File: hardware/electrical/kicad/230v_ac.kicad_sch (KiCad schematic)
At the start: 0 parts

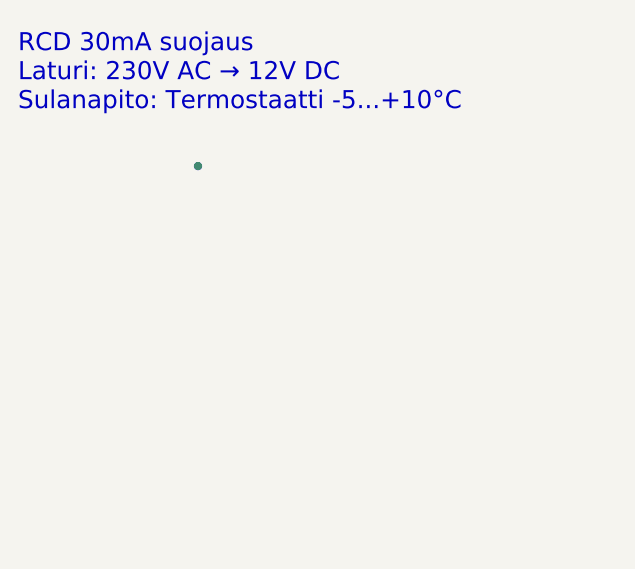
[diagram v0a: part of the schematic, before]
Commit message: Add untracked files and updates
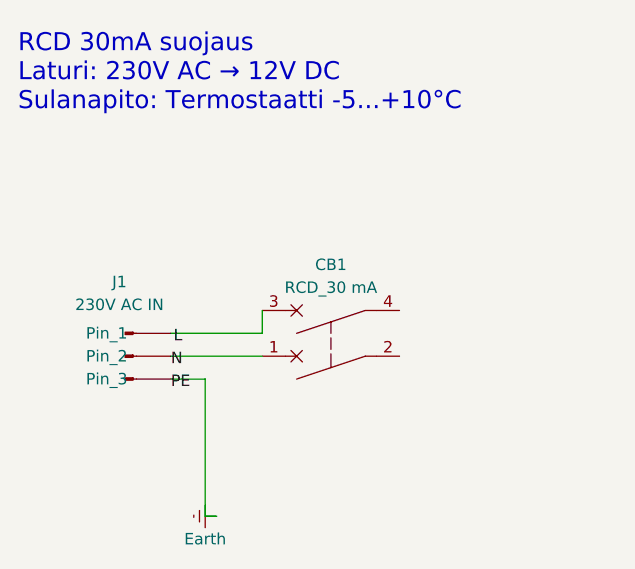
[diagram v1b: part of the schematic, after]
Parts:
- added CB1: RCD_30 mA, symbol Device:CircuitBreaker_2P
- added J1: 230V AC IN, symbol Connector:Conn_01x03_Pin
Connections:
- new net: CB1.1, J1.2 (Pin_2)
- new net: CB1.3, J1.1 (Pin_1)
- new net Earth: J1.3 (Pin_3)
